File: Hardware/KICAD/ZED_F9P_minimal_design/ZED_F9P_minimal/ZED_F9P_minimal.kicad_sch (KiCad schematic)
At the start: 21 parts, among them IC1 ZED-F9P-15B, J1 Conn_Coaxial_Small, U1 NCV8705ML33TCG

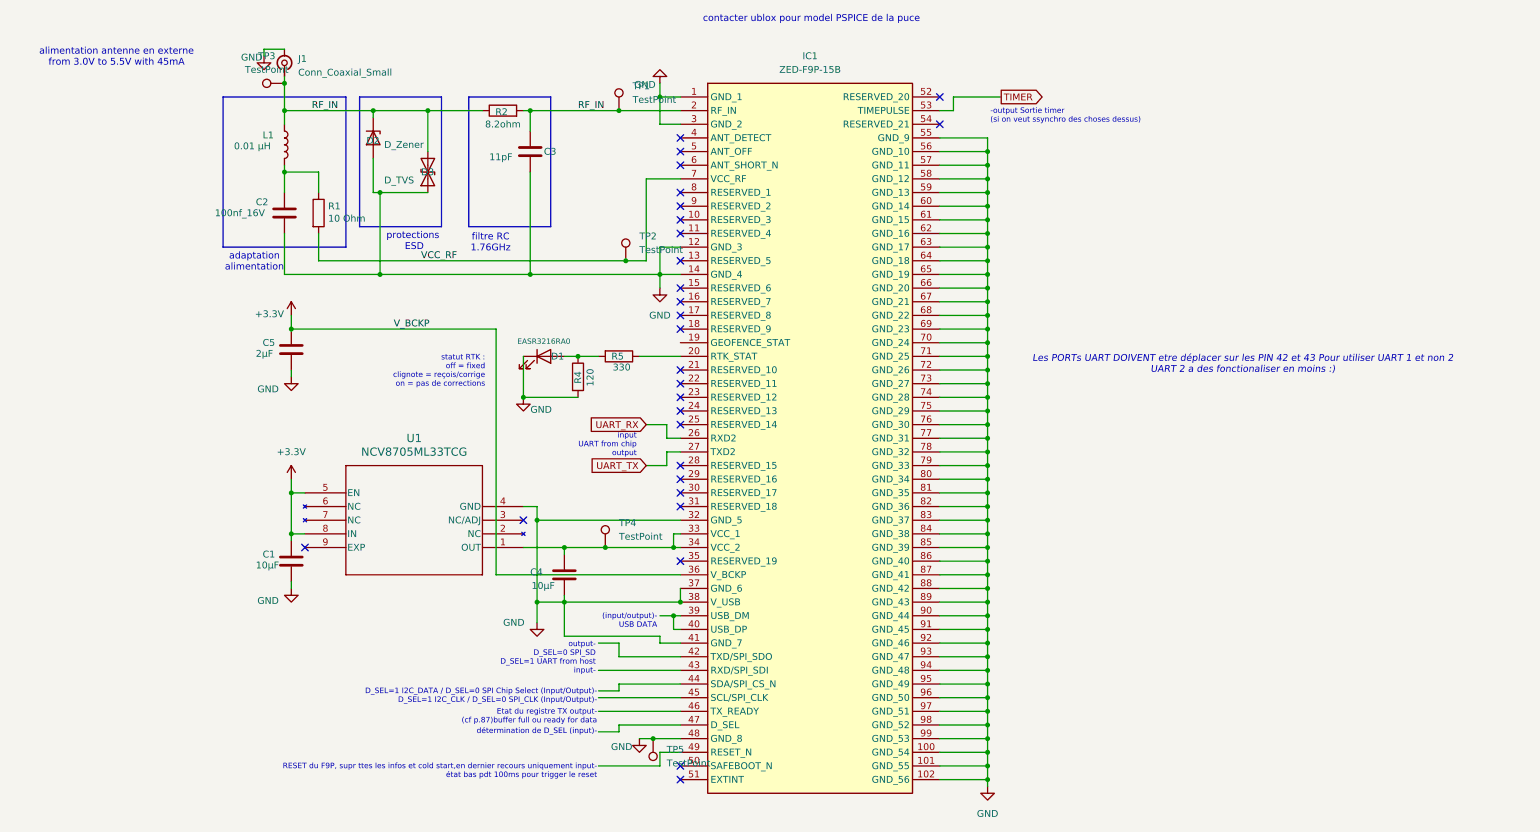
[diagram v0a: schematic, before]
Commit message: fix backup
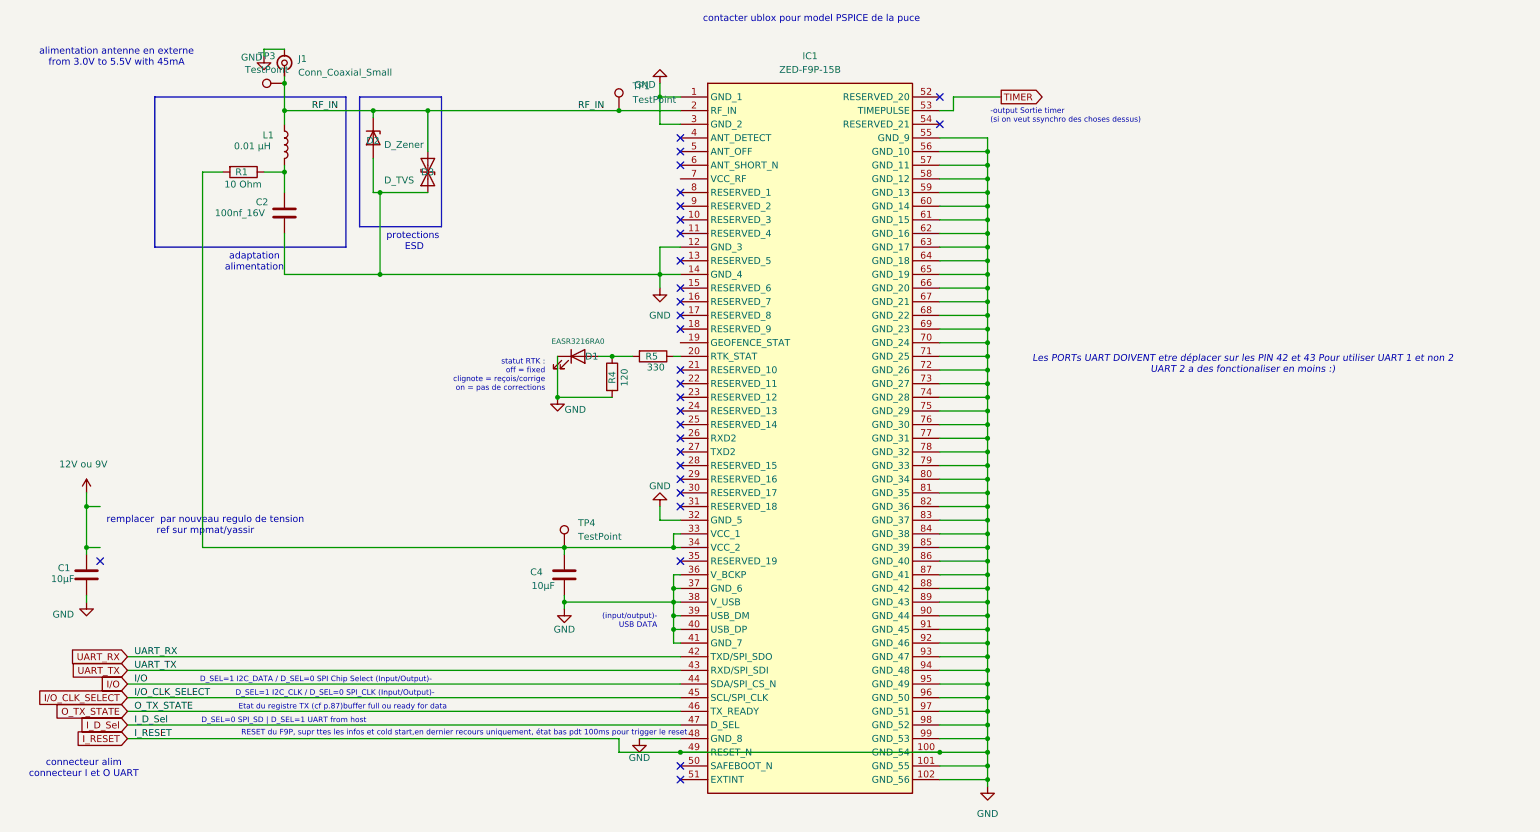
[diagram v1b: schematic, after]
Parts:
- removed C3: 11pF, 11pF:CAPC1608X90, symbol Device:C
- removed C5: 2µF, 2_2uF:CAPC1608X90, symbol Device:C
- removed R2: 8.2ohm, 10_Ohm:RC0402N_YAG, symbol Device:R
- removed TP2, TP5: TestPoint, symbol Connector:TestPoint
- removed U1: NCV8705ML33TCG, LM5168F:DFNW8-3x3_ONS, symbol Voltage regulator:NCV8705ML33TCG
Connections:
- net GND: now also IC1.36 (V_BCKP), IC1.39 (USB_DM), IC1.40 (USB_DP), IC1.49 (RESET_N)
- net UART_RX: now also IC1.42 (TXD/SPI_SDO); no longer IC1.26 (RXD2)
- net UART_TX: now also IC1.43 (RXD/SPI_SDI); no longer IC1.27 (TXD2)
- net at C4.1, IC1.33 (VCC_1), IC1.34 (VCC_2)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: now also R1.2
- net I/O : now reaches IC1.44 (SDA/SPI_CS_N)
- net I/O_CLK_SELECT: now reaches IC1.45 (SCL/SPI_CLK)
- net O_TX_STATE: now reaches IC1.46 (TX_READY)
- net I_D_Sel: now reaches IC1.47 (D_SEL)
- net +3.3V renamed 12V ou 9V
- net 12V ou 9V: no longer IC1.36 (V_BCKP)
- net VCC_RF: no longer names the net of IC1.7 (VCC_RF)
- net VCC_RF: no longer R1.2
- no-connect marks 28 -> 29
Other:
- note added: "D_SEL=0 SPI_SD | D_SEL=1 UART from host"
- note added: "D_SEL=1 I2C_CLK / D_SEL=0 SPI_CLK (Input/Output)-"
- note added: "D_SEL=1 I2C_DATA / D_SEL=0 SPI Chip Select (Input/Output)-"
- note added: "Etat du registre TX (cf p.87)buffer full ou ready for data"
- note added: "RESET du F9P, supr ttes les infos et cold start,en dernier recours uniquement, état bas pdt 100ms pour trigger le reset"
- note added: "connecteur alim connecteur I et O UART"
- note added: "remplacer par nouveau regulo de tension ref sur mpmat/yassir"
- note removed: "D_SEL=1 I2C_DATA / D_SEL=0 SPI Chip Select (Input/Output)- D_SEL=1 I2C_CLK / D_SEL=0 SPI_CLK (Input/Output)-"
- note removed: "Etat du registre TX output- (cf p.87)buffer full ou ready for data"
- note removed: "RESET du F9P, supr ttes les infos et cold start,en dernier recours uniquement input- état bas pdt 100ms pour trigger le reset"
- note removed: "détermination de D_SEL (input)-"
- note removed: "filtre RC 1.76GHz"
- note removed: "input UART from chip output"
- note removed: "output- D_SEL=0 SPI_SD D_SEL=1 UART from host input-"
- moved on the sheet: C1, D1, R1, R4, R5, TP4
